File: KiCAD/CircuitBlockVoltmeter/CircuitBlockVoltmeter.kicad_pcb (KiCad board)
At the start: 2 copper layers, 66 x 31.8 mm, 26 parts, among them J1 SSD1306_128x32_OLED, J3 Conn_01x02_Pin, SW1 SW_SPDT, U1 ATtiny85-20P, U4 OPA2340, U5 LM385BZ-2.5, U6 OPA2340

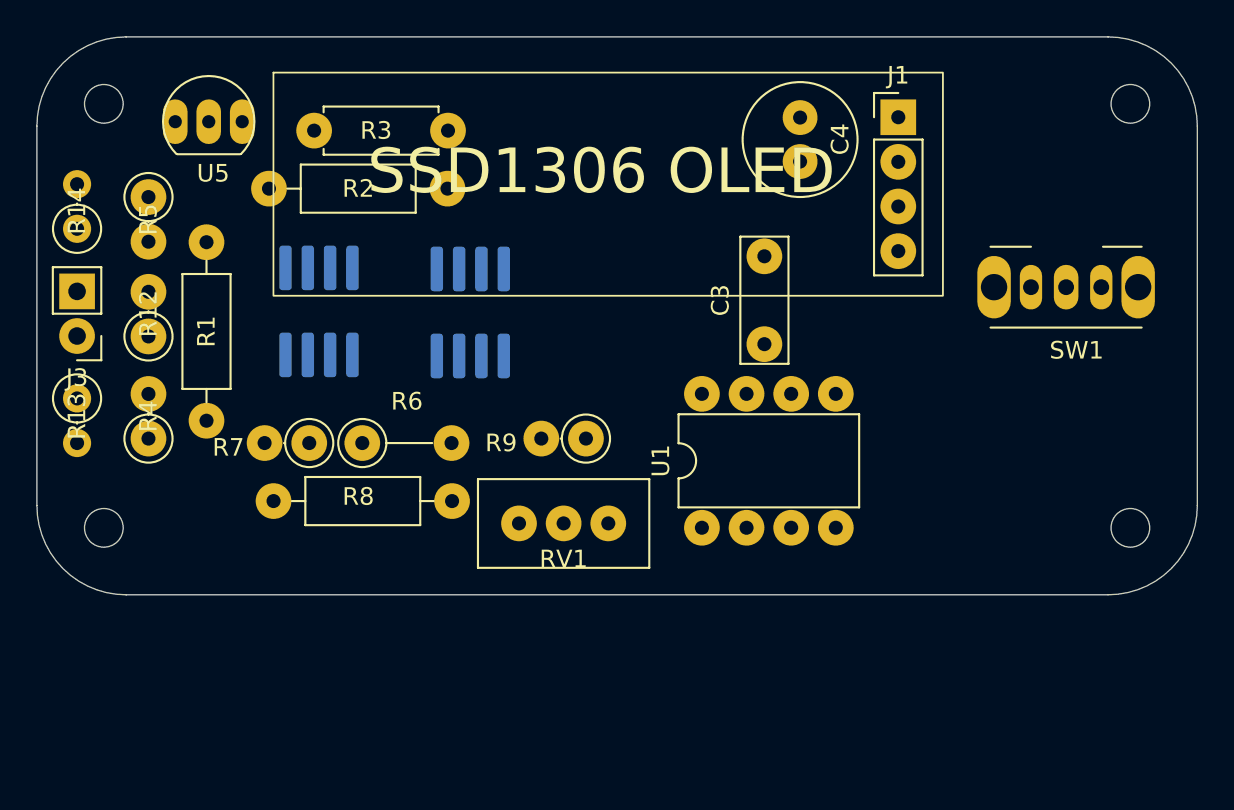
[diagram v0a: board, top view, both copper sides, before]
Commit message: Edit CAD
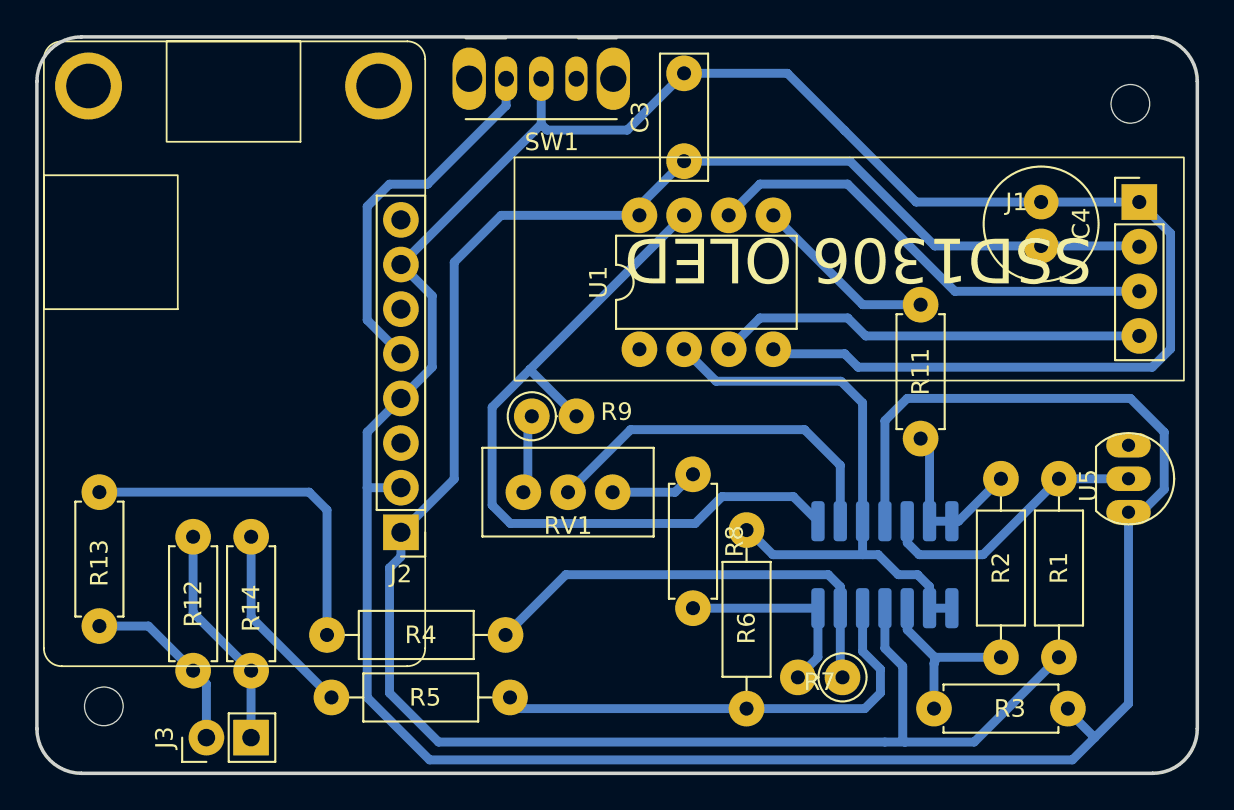
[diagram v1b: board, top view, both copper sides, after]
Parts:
- removed the REF** at (29.2, 53.3)
- removed the REF** at (87.6, 53.3)
- removed U4, U6: OPA2340, Package_SO:SOIC-8_3.9x4.9mm_P1.27mm
- added J2: PowerBoost_500C, User:PowerBoost 500C, F.Cu at (46.1, 53.6)
- added R11: 0, Resistor_THT:R_Axial_DIN0207_L6.3mm_D2.5mm_P7.62mm_Horizontal, F.Cu at (75.7, 40.6)
- added U2: OPA4340UA, Package_SO:SOIC-14_3.9x8.7mm_P1.27mm, B.Cu at (73.7, 55.4)
- R12, R13, R14: footprint Resistor_THT:R_Axial_DIN0207_L6.3mm_D2.5mm_P2.54mm_Vertical -> Resistor_THT:R_Axial_DIN0207_L6.3mm_D2.5mm_P7.62mm_Horizontal
- R4, R5: footprint Resistor_THT:R_Axial_DIN0207_L6.3mm_D2.5mm_P2.54mm_Vertical -> Resistor_THT:R_Axial_DIN0207_L6.3mm_D2.5mm_P10.16mm_Horizontal
- R6: footprint Resistor_THT:R_Axial_DIN0207_L6.3mm_D2.5mm_P5.08mm_Vertical -> Resistor_THT:R_Axial_DIN0207_L6.3mm_D2.5mm_P10.16mm_Horizontal
- R8: footprint Resistor_THT:R_Axial_DIN0207_L6.3mm_D2.5mm_P10.16mm_Horizontal -> Resistor_THT:R_Axial_DIN0207_L6.3mm_D2.5mm_P7.62mm_Horizontal
- moved U5 56.9 mm to (87.5, 49.3), turned to -90 degrees
- moved R1 50.3 mm to (83.6, 60.7)
- moved R2 44.8 mm to (80.3, 50.5), turned to -90 degrees
- moved R3 43.0 mm to (76.5, 63.6), turned to 0 degrees
- moved REF** 34.3 mm to (29.2, 63.5)
- moved R7 33.1 mm to (71.2, 61.8)
- moved SW1 32.1 mm to (56.1, 27.8)
- moved R5 30.3 mm to (42.2, 63.0), turned to 0 degrees
- moved R14 27.0 mm to (37.6, 61.5)
- moved R6 26.6 mm to (65.8, 63.6), turned to 90 degrees
- moved J3 24.0 mm to (35.0, 65.3), turned to 90 degrees
- moved R12 19.2 mm to (34.3, 61.5)
- moved R4 15.1 mm to (41.9, 59.4), turned to 0 degrees
- moved J1 14.5 mm to (88.1, 34.8)
- moved C4 14.5 mm to (82.5, 37.3)
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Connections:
- SW1 pad 2: Net-(J2-Pin_5) -> GND
- SW1 pad 3: GND -> Net-(J2-EN)
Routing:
- net GND: track 0.00 -> 201.4 mm
- net +5V: track 0.00 -> 119.1 mm
- net AIN: track 0.00 -> 45.0 mm
- net AGND: track 0.00 -> 33.3 mm
- net Net-(U2B-+): track 0.00 -> 27.0 mm
- net SCL: track 0.00 -> 26.6 mm
- net Net-(U2B--): track 0.00 -> 26.0 mm
- net SDA: track 0.00 -> 24.5 mm
- net Net-(U2C--): track 0.00 -> 21.0 mm
- net Net-(J2-EN): track 0.00 -> 20.6 mm
- net Net-(R13-Pad2): track 0.00 -> 20.5 mm
- net AREF: track 0.00 -> 20.5 mm
- net Net-(U2D-+): track 0.00 -> 15.9 mm
- net Net-(J3-Pin_2): track 0.00 -> 12.9 mm
- net Net-(R7-Pad2): track 0.00 -> 11.5 mm
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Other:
- board size 66 x 31.8 mm -> 66 x 41.9 mm
